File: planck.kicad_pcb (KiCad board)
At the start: 2 copper layers, 53 parts, among them J1 USB_C_Receptacle_USB2.0, K1 KEYSW, K2 KEYSW, K3 KEYSW, K4 KEYSW, SW1 SW_PUSH, U1 ATmega32U4-M, Y1 Crystal_GND24_Small

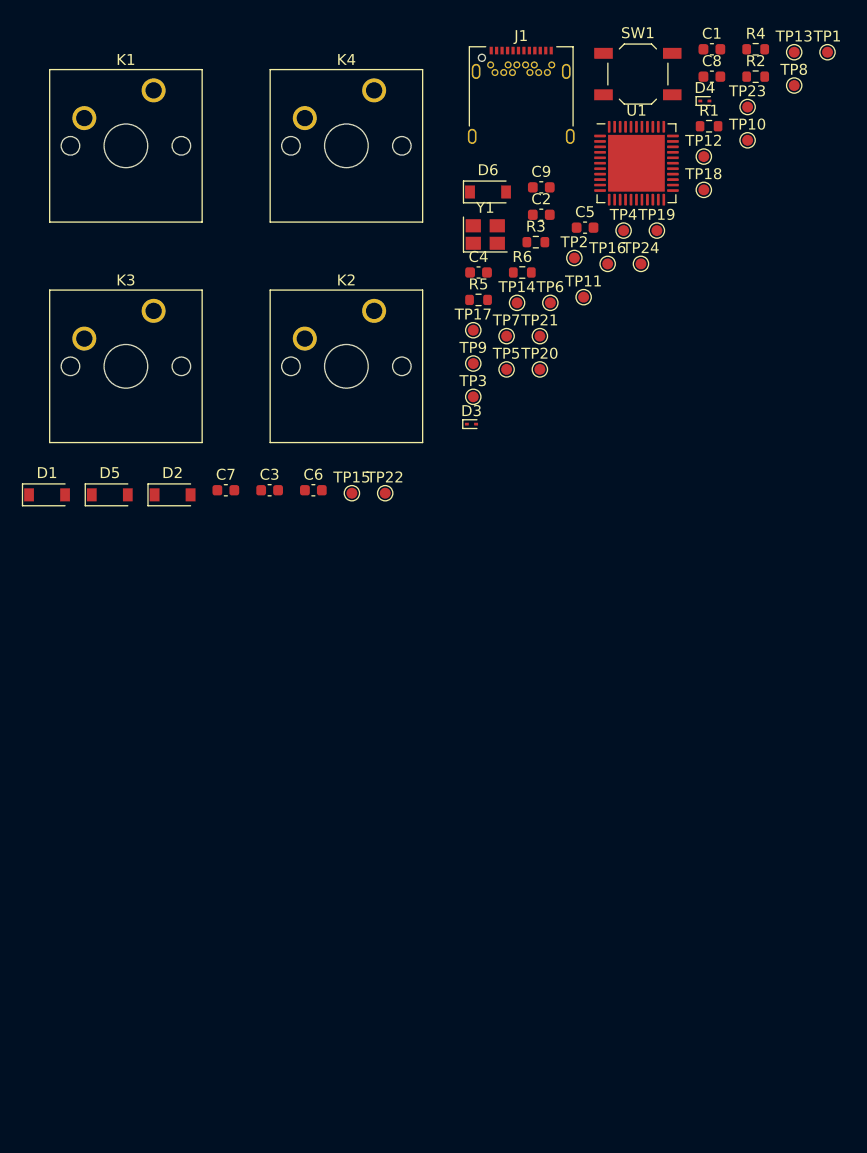
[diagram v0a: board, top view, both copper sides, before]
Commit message: poured fills
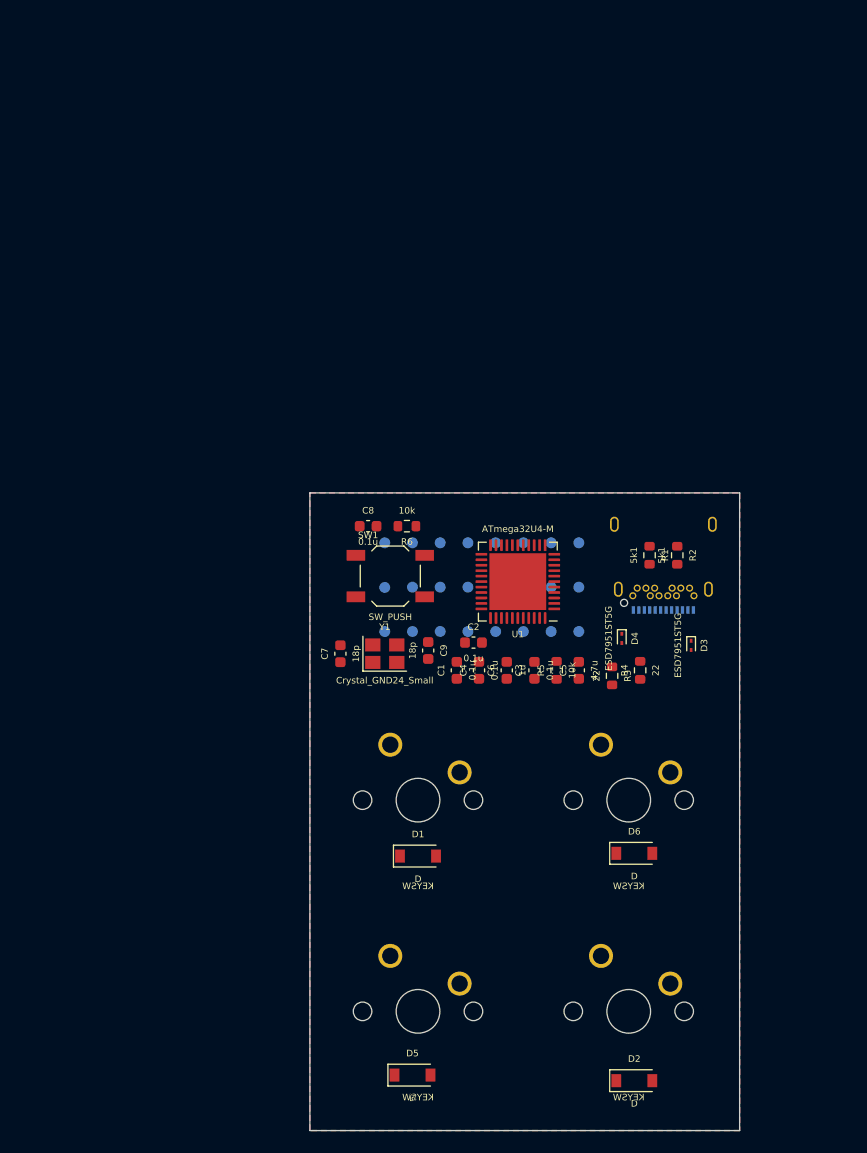
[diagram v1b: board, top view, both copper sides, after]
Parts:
- J1, K1, K2, K3, K4, TP1, TP2: moved to B.Cu
- TP10: value TestPoint -> PB5; moved to B.Cu
- TP11: value TestPoint -> PB6; moved to B.Cu
- TP12: value TestPoint -> PB7; moved to B.Cu
- TP13: value TestPoint -> PC6; moved to B.Cu
- TP14: value TestPoint -> PC7; moved to B.Cu
- TP15: value TestPoint -> PD0; moved to B.Cu
- TP16: value TestPoint -> PD1; moved to B.Cu
- TP17: value TestPoint -> PD2; moved to B.Cu
- TP18: value TestPoint -> PD3; moved to B.Cu
- TP19: value TestPoint -> PD4; moved to B.Cu
- TP20: value TestPoint -> PD6; moved to B.Cu
- TP21: value TestPoint -> PD7; moved to B.Cu
- TP22: value TestPoint -> PE6; moved to B.Cu
- TP23: value TestPoint -> PF6; moved to B.Cu
- TP24: value TestPoint -> PF7; moved to B.Cu
- TP3: value TestPoint -> AREF; moved to B.Cu
- TP4: value TestPoint -> PD5; moved to B.Cu
- TP5: value TestPoint -> PB0; moved to B.Cu
- TP6: value TestPoint -> PB1; moved to B.Cu
- TP7: value TestPoint -> PB2; moved to B.Cu
- TP8: value TestPoint -> PB3; moved to B.Cu
- TP9: value TestPoint -> PB4; moved to B.Cu
- moved D2 68.3 mm to (107.2, 132.6)
- moved K1 63.7 mm to (84.8, 101.8), turned to 180 degrees
- moved K4 63.4 mm to (104.1, 101.8), turned to 180 degrees
- moved K3 62.9 mm to (84.8, 121.2), turned to 180 degrees
- moved K2 62.6 mm to (104.1, 121.2), turned to 180 degrees
- moved D6 62.1 mm to (107.2, 111.8)
- moved C1 61.5 mm to (90.9, 95.0), turned to 90 degrees
- moved D5 60.0 mm to (86.9, 132.1)
- moved R4 57.9 mm to (107.7, 95.0), turned to 90 degrees
- moved TP13 56.1 mm to (94.5, 87.4), turned to 180 degrees
- moved TP1 55.2 mm to (99.6, 87.4), turned to 180 degrees
- moved TP23 53.6 mm to (86.9, 87.4), turned to 180 degrees
- moved C8 51.8 mm to (82.8, 81.8)
- moved SW1 51.3 mm to (84.8, 86.4)
- moved TP8 50.0 mm to (94.5, 83.3), turned to 180 degrees
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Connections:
- net /reset renamed /~{reset}
- net Net-(TP10-Pad1) renamed /PB5
- net Net-(TP11-Pad1) renamed /PB6
- net Net-(TP12-Pad1) renamed /PB7
- net Net-(TP13-Pad1) renamed /PC6
- net Net-(TP14-Pad1) renamed /PC7
- net Net-(TP15-Pad1) renamed /PD0
- net Net-(TP16-Pad1) renamed /PD1
- net Net-(TP17-Pad1) renamed /PD2
- net Net-(TP18-Pad1) renamed /PD3
- net Net-(TP19-Pad1) renamed /PD4
- net Net-(TP20-Pad1) renamed /PD6
- net Net-(TP21-Pad1) renamed /PD7
- net Net-(TP22-Pad1) renamed /PE6
- net Net-(TP23-Pad1) renamed /PF6
- net Net-(TP24-Pad1) renamed /PF7
- net Net-(TP4-Pad1) renamed /PD5
- net Net-(TP5-Pad1) renamed /PB0
- net Net-(TP6-Pad1) renamed /PB1
- net Net-(TP7-Pad1) renamed /PB2
- net Net-(TP8-Pad1) renamed /PB3
- net Net-(TP9-Pad1) renamed /PB4
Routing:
- added copper zone on B.Cu, net GND
- added copper zone on F.Cu, net GND
- added copper zone on In1.Cu, net GND
- added copper zone on In2.Cu, net VCC
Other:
- board outline added: 39.4 x 58.4 mm
- copper layers 2 -> 4
